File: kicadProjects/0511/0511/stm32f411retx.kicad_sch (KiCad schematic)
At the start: 16 parts, among them U8 STM32F411RETx

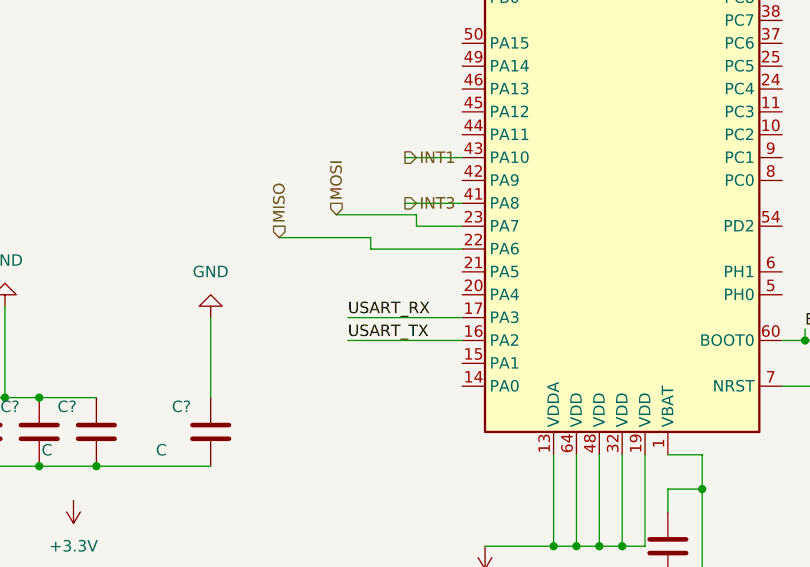
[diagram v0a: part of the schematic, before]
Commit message: poursuite
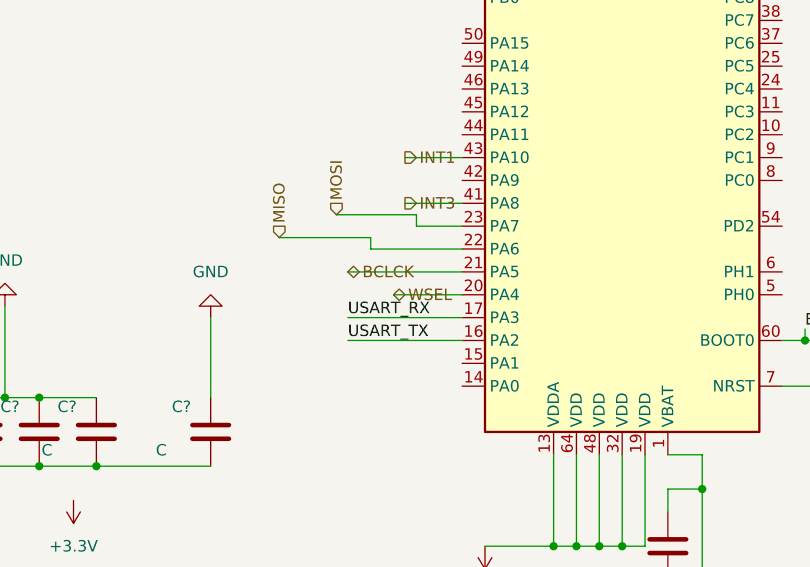
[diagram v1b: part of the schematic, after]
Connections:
- net WSEL: now reaches U8.20 (PA4)
- net BCLCK: now reaches U8.21 (PA5)
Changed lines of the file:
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@@
+	(wire
+		(pts
+			(xy 73.66 116.84) (xy 81.28 116.84)
+		)
+		(stroke
+			(width 0)
+			(type default)
+		)
+	)
 	(wire
 		(pts
@@
 		(pts
 			(xy 104.14 138.43) (xy 104.14 140.97)
+		)
+		(stroke
+			(width 0)
+			(type default)
+		)
+	)
+	(wire
+		(pts
+			(xy 68.58 114.3) (xy 81.28 114.3)
 		)
 		(stroke
@@
 		)
 	)
+	(hierarchical_label "WSEL"
+		(shape bidirectional)
+		(at 73.66 116.84 0)
+		(effects
+			(font
+				(size 1.27 1.27)
+			)
+			(justify left)
+		)
+	)
 	(hierarchical_label "INT2"
 		(shape output)
@@
 		(effects
 			(font
+				(size 1.27 1.27)
+			)
+			(justify left)
+		)
+	)
+	(hierarchical_label "BCLCK"
+		(shape bidirectional)
+		(at 68.58 114.3 0)
+		(effects
+			(font
